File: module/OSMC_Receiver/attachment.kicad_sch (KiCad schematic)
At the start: 8 parts, among them U13 OSMC Module Board, U14 OSMC Module Board, U15 OSMC Module Board, U16 OSMC Module Board, U17 OSMC Module Board, U18 OSMC Module Board, U19 OSMC Module Board, U20 OSMC Module Board

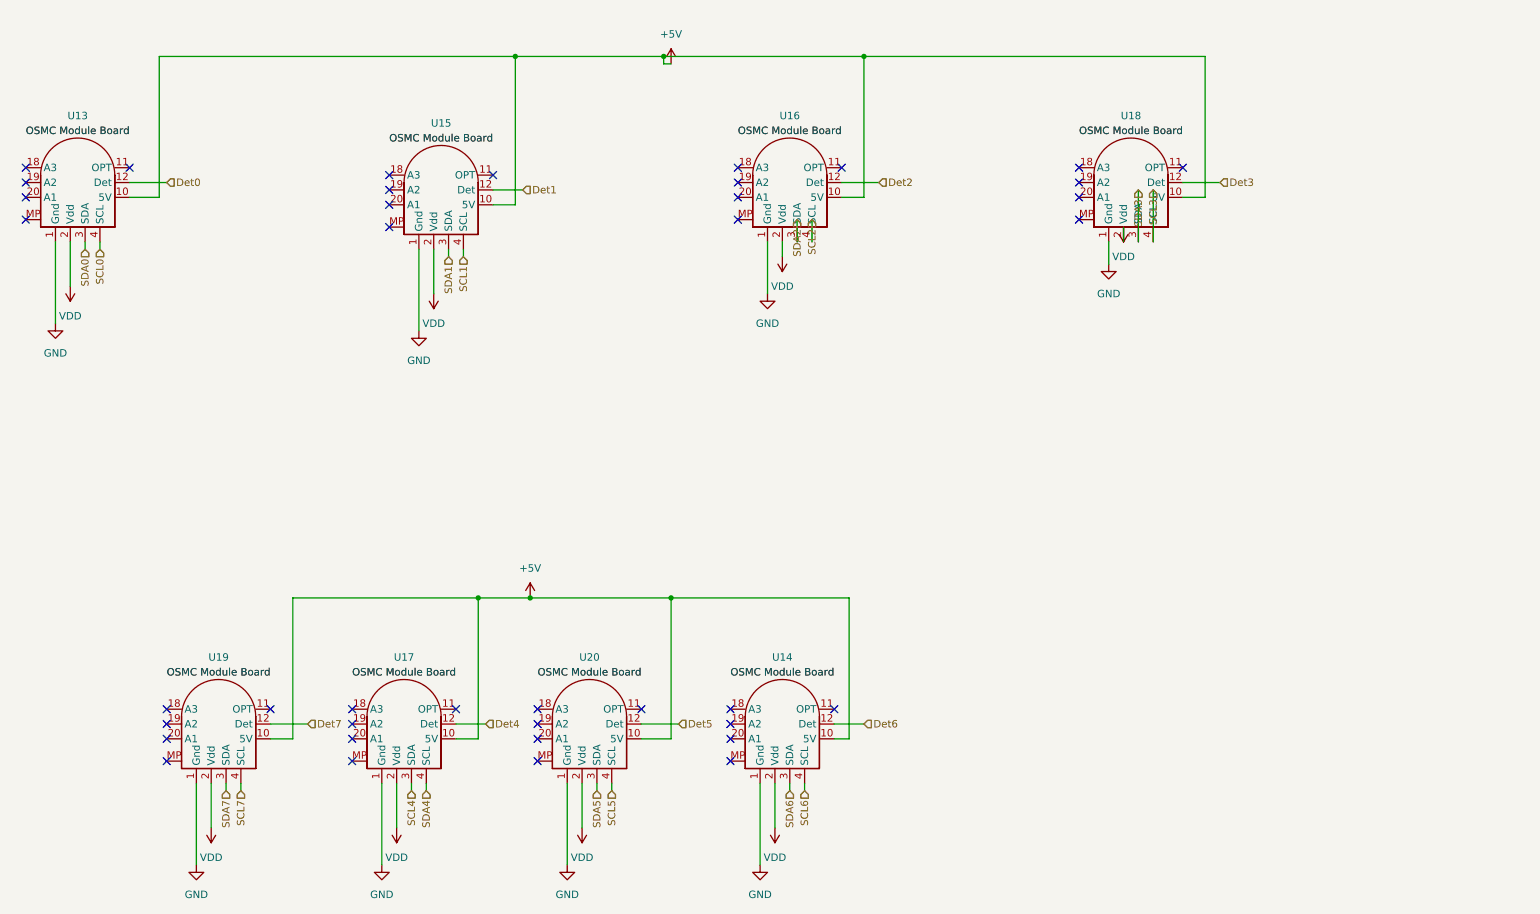
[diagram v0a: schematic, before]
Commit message: reviewed PCBs
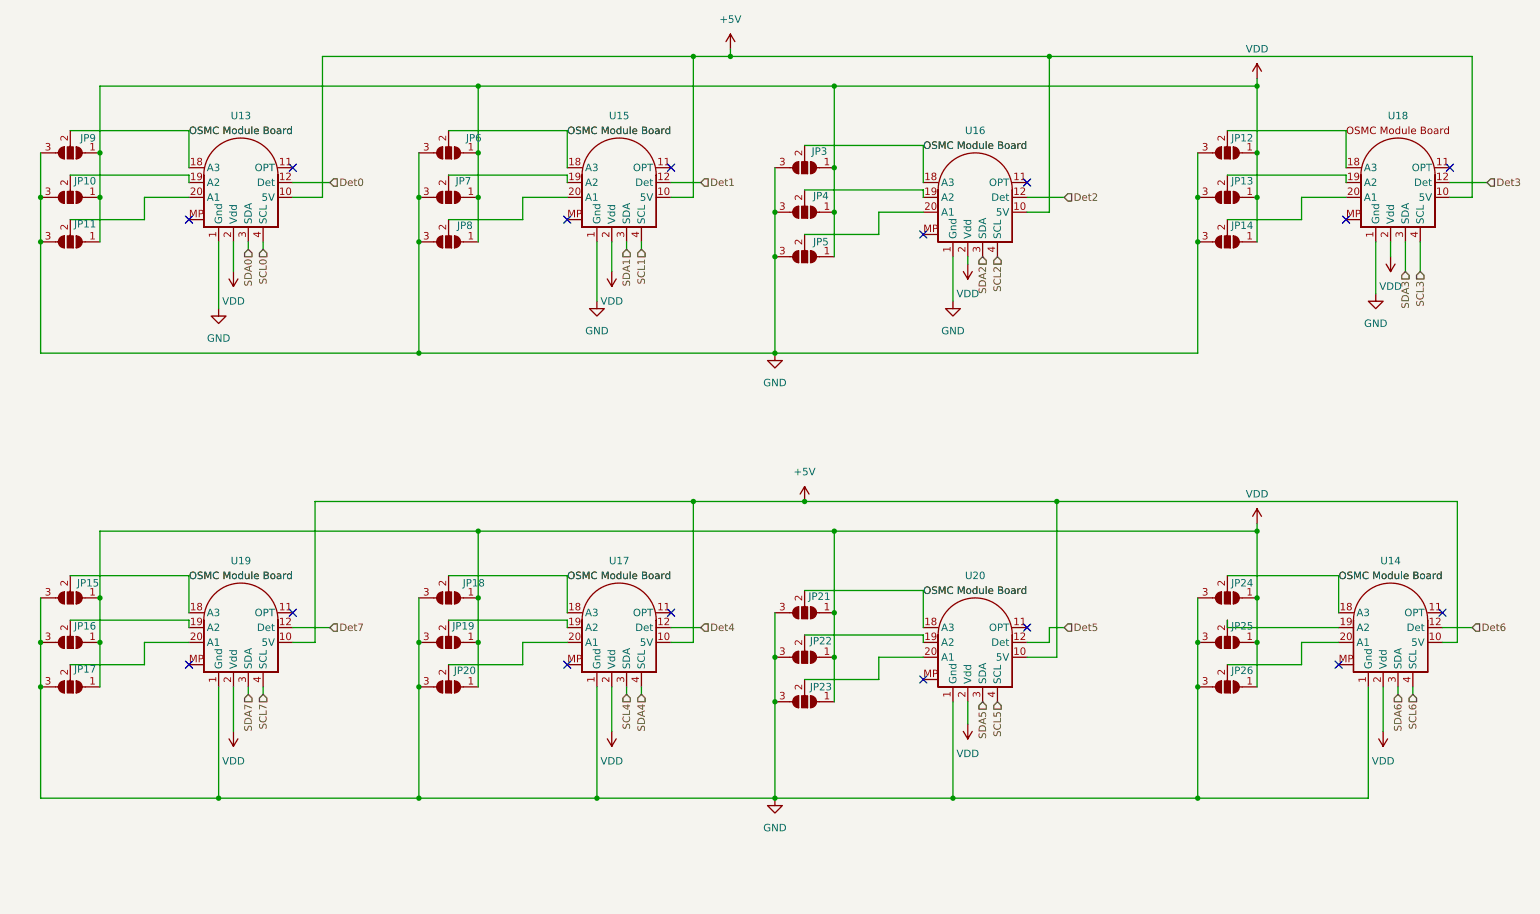
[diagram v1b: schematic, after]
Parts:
- added JP10, JP11, JP12, JP13, JP14, JP15, JP16, JP17, JP18, JP19, JP20, JP21, JP22, JP23, JP24, JP25, JP26, JP3, JP4, JP5, JP6, JP7, JP8, JP9: SolderJumper_3_Open, Jumper:SolderJumper-3_P1.3mm_Open_Pad1.0x1.5mm, symbol Jumper:SolderJumper_3_Open
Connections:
- net GND: now also JP10.3 (B), JP11.3 (B), JP12.3 (B), JP13.3 (B), JP14.3 (B), JP15.3 (B), JP16.3 (B), JP17.3 (B), JP18.3 (B), JP19.3 (B), JP20.3 (B), JP21.3 (B), JP22.3 (B), JP23.3 (B), JP24.3 (B), JP25.3 (B), JP26.3 (B), JP3.3 (B), JP4.3 (B), JP5.3 (B), JP6.3 (B), JP7.3 (B), JP8.3 (B), JP9.3 (B)
- net VDD: now also JP10.1 (A), JP11.1 (A), JP12.1 (A), JP13.1 (A), JP14.1 (A), JP15.1 (A), JP16.1 (A), JP17.1 (A), JP18.1 (A), JP19.1 (A), JP20.1 (A), JP21.1 (A), JP22.1 (A), JP23.1 (A), JP24.1 (A), JP25.1 (A), JP26.1 (A), JP3.1 (A), JP4.1 (A), JP5.1 (A), JP6.1 (A), JP7.1 (A), JP8.1 (A), JP9.1 (A)
- net at U19.18 (A3): now also JP15.2 (C)
- net at U19.19 (A2): now also JP16.2 (C)
- net at U19.20 (A1): now also JP17.2 (C)
- net at U17.18 (A3): now also JP18.2 (C)
- net at U17.19 (A2): now also JP19.2 (C)
- net at U17.20 (A1): now also JP20.2 (C)
- net at U15.18 (A3): now also JP6.2 (C)
- net at U15.19 (A2): now also JP7.2 (C)
- net at U15.20 (A1): now also JP8.2 (C)
- net at U18.18 (A3): now also JP12.2 (C)
- net at U18.19 (A2): now also JP13.2 (C)
- net at U18.20 (A1): now also JP14.2 (C)
- net at U13.18 (A3): now also JP9.2 (C)
- net at U13.19 (A2): now also JP10.2 (C)
- net at U13.20 (A1): now also JP11.2 (C)
- net at U20.18 (A3): now also JP21.2 (C)
- net at U20.19 (A2): now also JP22.2 (C)
- net at U20.20 (A1): now also JP23.2 (C)
- net at U14.18 (A3): now also JP24.2 (C)
- net at U14.19 (A2): now also JP25.2 (C)
- net at U14.20 (A1): now also JP26.2 (C)
- net at U16.18 (A3): now also JP3.2 (C)
- net at U16.19 (A2): now also JP4.2 (C)
- net at U16.20 (A1): now also JP5.2 (C)
- no-connect marks 40 -> 16
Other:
- moved on the sheet: U13, U14, U15, U16, U17, U18, U19, U20
